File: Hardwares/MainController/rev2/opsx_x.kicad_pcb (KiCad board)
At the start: 2 copper layers, 95.9 x 27.8 mm, 62 parts, among them J1 Conn_01x02, J3 Conn_01x02, Q1 Q_NMOS_GSD, Q2 Q_NMOS_GSD, Q3 Q_PMOS_GSD, Q4 MMBT3904, U1 RP2040, U2 TLV70433DBVR, U3 W25Q128JVS, U4 OPTICAL-TSL2561T(6P-3.8X2.6MM), Y1 Crystal_GND2

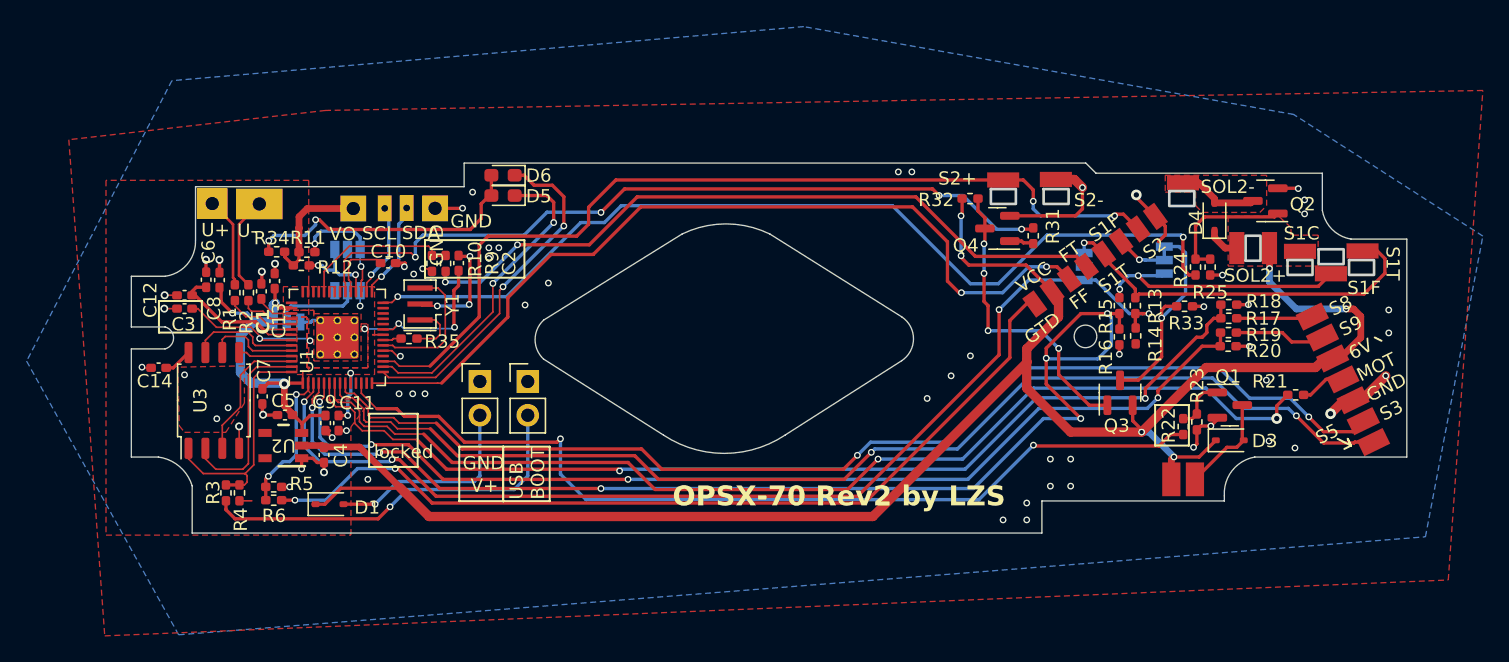
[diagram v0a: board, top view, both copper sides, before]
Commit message: 声纳工作正常
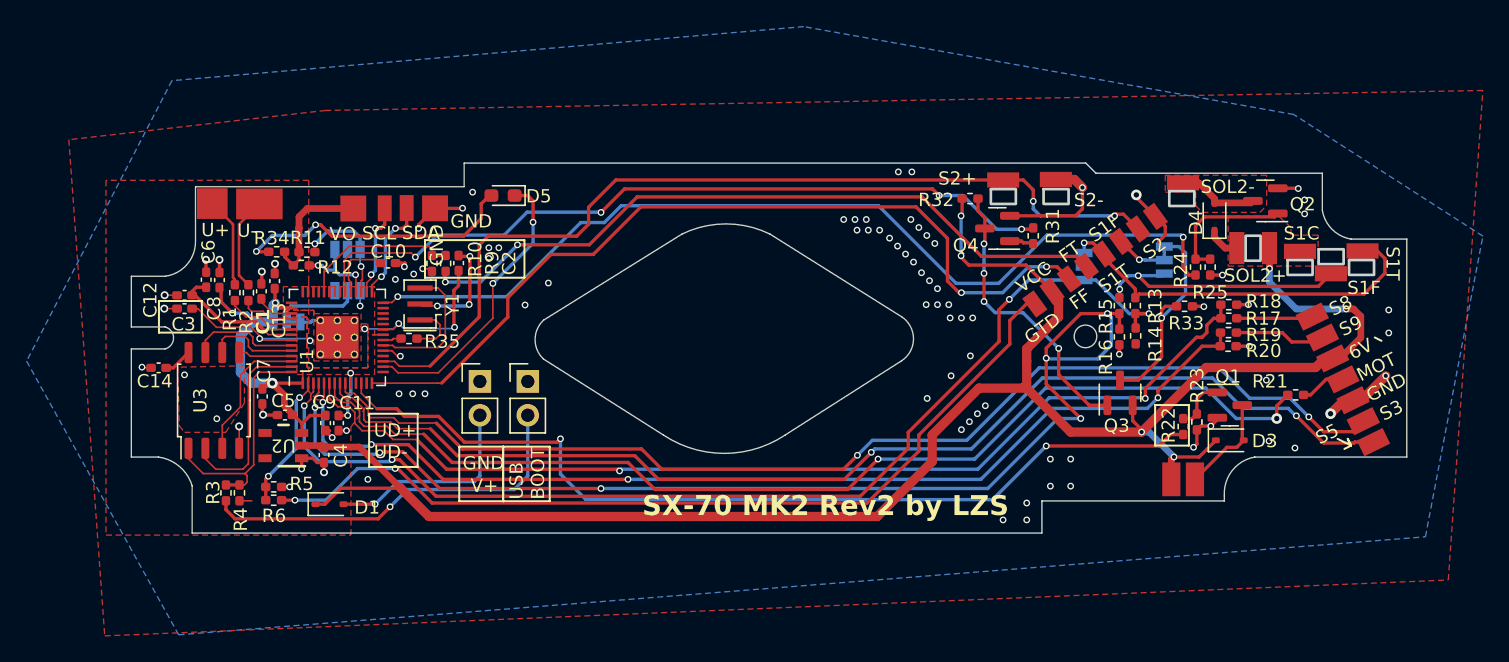
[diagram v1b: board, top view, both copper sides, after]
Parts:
- removed D6: LED, Diode_SMD:D_0603_1608Metric_Pad1.05x0.95mm_HandSolder
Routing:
- net /LED2: track 26.1 -> 0.00 mm, vias 2 -> 0
- net GND: track 71.8 -> 73.8 mm, vias 66 -> 95
- net /LED1: track 23.6 -> 21.8 mm
- net Net-(Q3-G): track 22.8 -> 21.6 mm
- net /S1F_PF_MCU: track 58.7 -> 58.1 mm
- net /GTD-3: track 10.8 -> 10.2 mm
- net /SDA1: track 7.42 -> 7.76 mm, vias 1 -> 2
- net /SCL1: track 7.08 -> 7.06 mm, vias 1 -> 2
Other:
- board text added: "SX-70 MK2 Rev2 by LZS"
- board text added: "UD+ UD-"
- board text removed: "OPSX-70 Rev2 by LZS"
- board text removed: "locked"
